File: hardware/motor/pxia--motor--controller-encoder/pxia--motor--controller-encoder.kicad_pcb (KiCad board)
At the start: 2 copper layers, 42 x 42 mm, 10 parts, among them J1 IDC(CTRL>), J2 GPIO+PWR, U1 MT8512AT

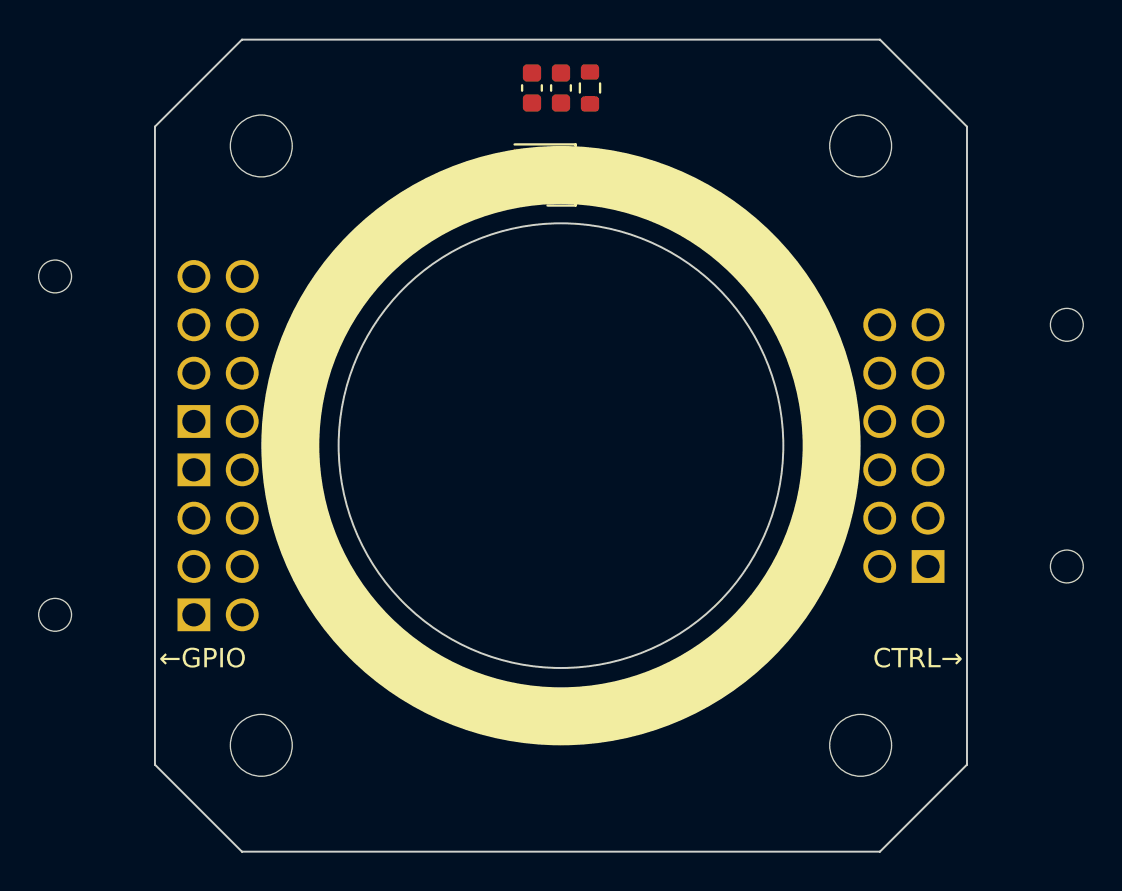
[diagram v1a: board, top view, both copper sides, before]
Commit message: finished routing
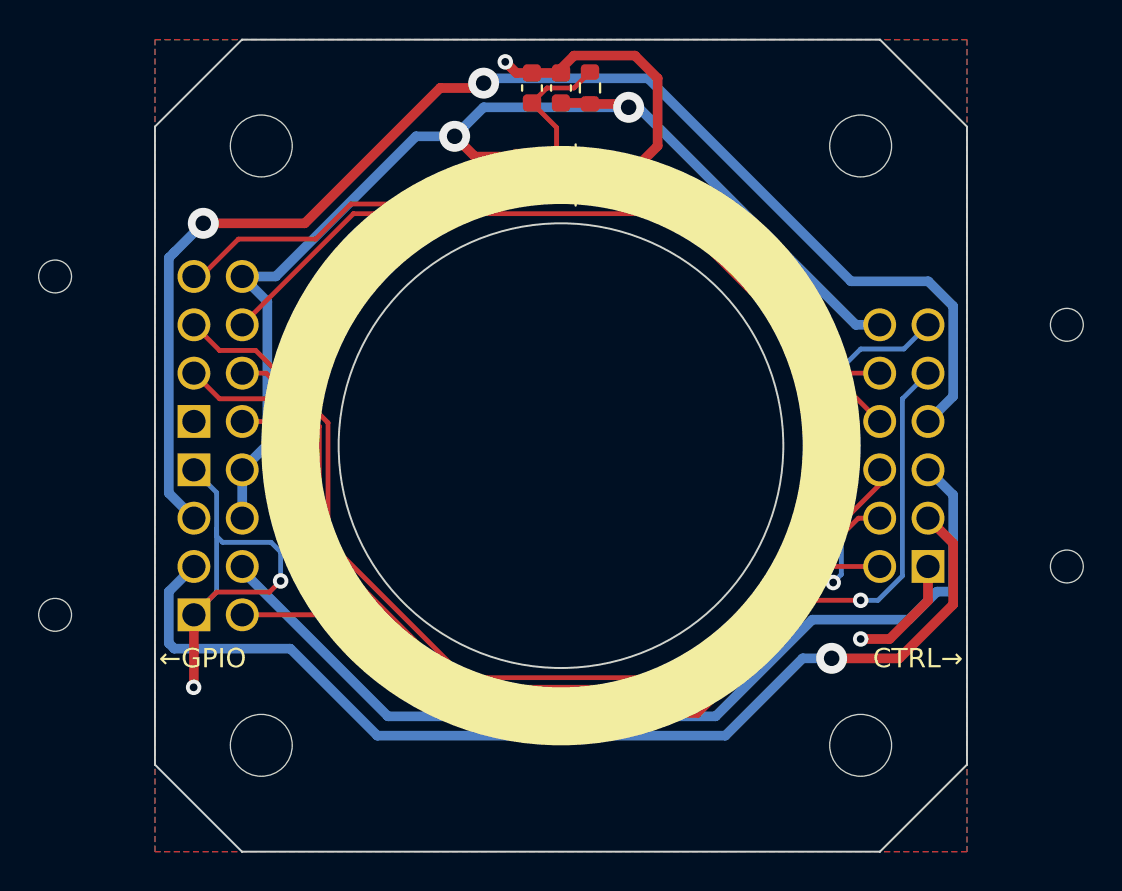
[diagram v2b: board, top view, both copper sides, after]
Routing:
- net /OUTPUT_1: track 0.00 -> 69.9 mm, vias 0 -> 2
- net +5V: track 0.00 -> 62.9 mm, vias 0 -> 2
- net /INPUT_6: track 0.00 -> 59.5 mm, vias 0 -> 1
- net /OUTPUT_3: track 0.00 -> 54.9 mm, vias 0 -> 1
- net /INPUT_3: track 0.00 -> 51.5 mm
- net /INPUT_1: track 0.00 -> 50.5 mm
- net /ANALOG_IN: track 0.00 -> 50.3 mm, vias 0 -> 1
- net /OUTPUT_2: track 0.00 -> 49.6 mm
- net /INPUT_5: track 0.00 -> 48.7 mm
- net /INPUT_4: track 0.00 -> 46.9 mm
- net GND: track 0.00 -> 45.8 mm, vias 0 -> 5
- net /INPUT_2: track 0.00 -> 39.8 mm
- added copper zone on F.Cu, net (none)
- added copper zone on B.Cu, net GND
